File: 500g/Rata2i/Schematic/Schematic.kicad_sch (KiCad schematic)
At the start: 33 parts, among them J1 Screw_Terminal_01x03, J10 Conn_01x03_Pin, J2 Screw_Terminal_01x03, J3 Screw_Terminal_01x03, J4 Screw_Terminal_01x03, J5 Screw_Terminal_01x03, J6 Screw_Terminal_01x03, J7 Battery, J8 Screw_Terminal_01x02, J9 Screw_Terminal_01x02, SW1 SW_SPDT, U1 DEV-16771, U2 TB6612FNG, U3 R-78K5.0-0.5, U4 R-78K5.0-0.5

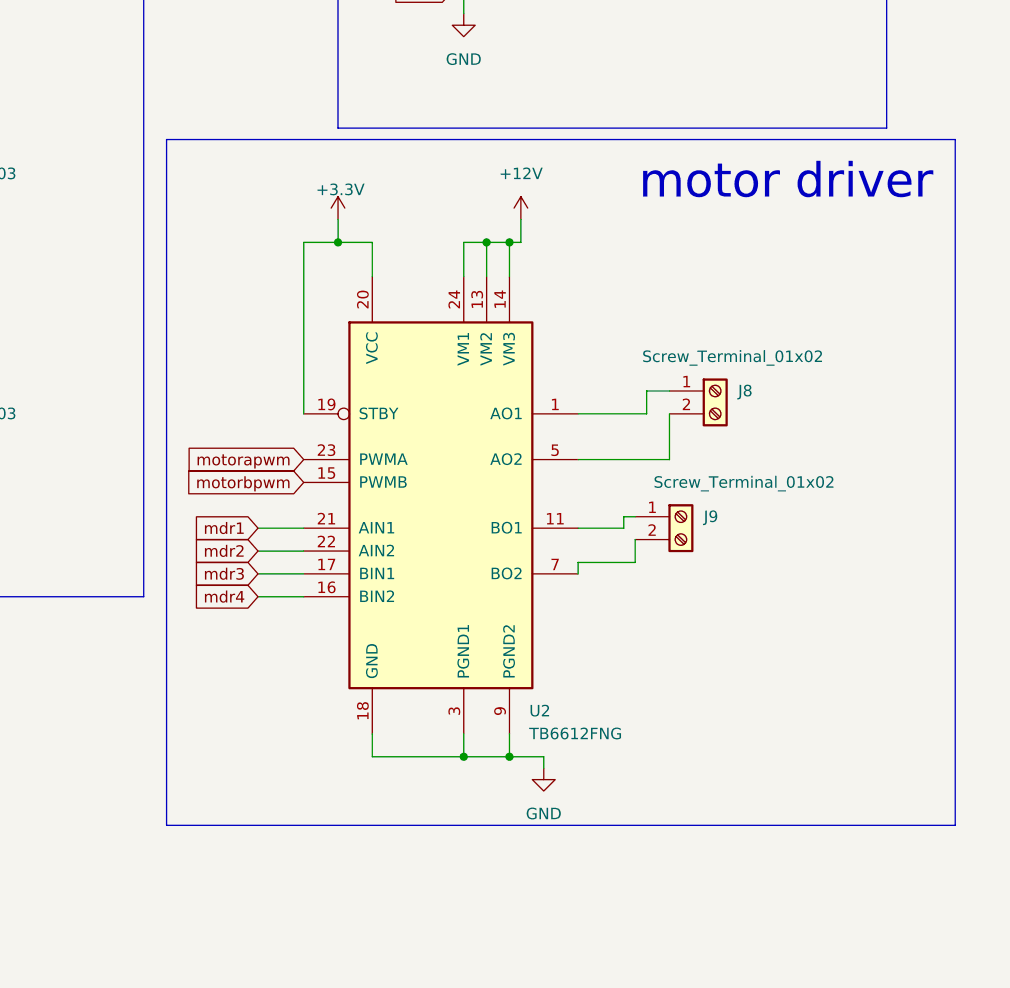
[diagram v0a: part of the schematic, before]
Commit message: PCB extravaganza
pcb update
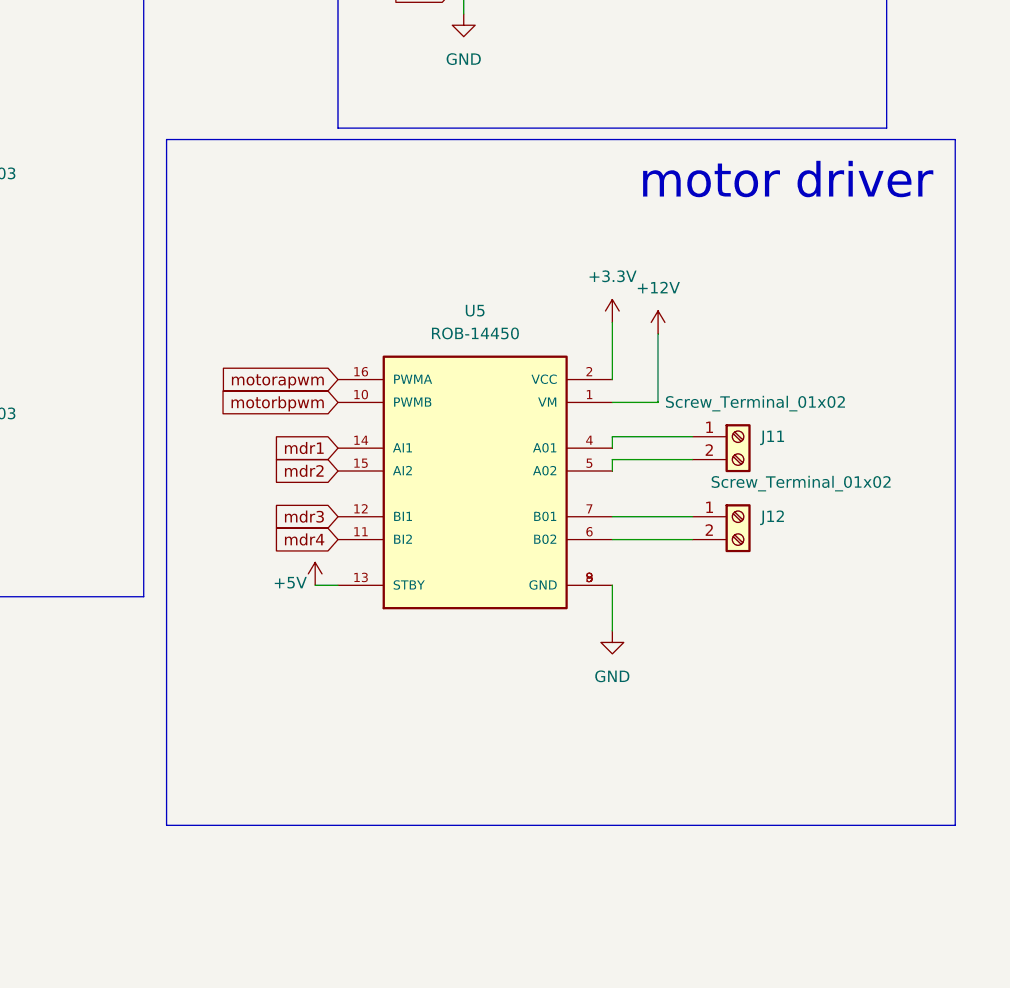
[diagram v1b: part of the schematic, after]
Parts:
- removed J8, J9: Screw_Terminal_01x02, robowrestling:Screw Terminal, symbol Connector:Screw_Terminal_01x02
- removed U2: TB6612FNG, Package_SO:SSOP-24_5.3x8.2mm_P0.65mm, symbol Driver_Motor:TB6612FNG
- added J11, J12: Screw_Terminal_01x02, TerminalBlock:TerminalBlock_Xinya_XY308-2.54-2P_1x02_P2.54mm_Horizontal, symbol Connector:Screw_Terminal_01x02
- added U5: ROB-14450, robowrestling:MOTOR_DRIVER, symbol motor driver:ROB-14450
- J1, J2, J3, J4, J5, J6: footprint Connector_PinHeader_2.54mm:PinHeader_1x03_P2.54mm_Vertical -> TerminalBlock:TerminalBlock_Xinya_XY308-2.54-3P_1x03_P2.54mm_Horizontal
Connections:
- net +12V: now also U5.1 (VM)
- net +3.3V: now also U5.2 (VCC)
- net +5V: now also U5.13 (STBY)
- net GND: now also U5.3 (GND), U5.8 (GND), U5.9 (GND)
- net mdr1: now also U5.14 (AI1)
- net mdr2: now also U5.15 (AI2)
- net mdr3: now also U5.12 (BI1)
- net mdr4: now also U5.11 (BI2)
- net motorapwm: now also U5.16 (PWMA)
- net motorbpwm: now also U5.10 (PWMB)
- new net: J11.1 (Pin_1), U5.4 (A01)
- new net: J11.2 (Pin_2), U5.5 (A02)
- new net: J12.2 (Pin_2), U5.6 (B02)
- new net: J12.1 (Pin_1), U5.7 (B01)
